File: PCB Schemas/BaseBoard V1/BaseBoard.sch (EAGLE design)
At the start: 31 parts, among them IC1 74HC595D, IC2 74HC595D, IC3 74HC595D, U1 ATMEGA2560AU, X1 16MHz

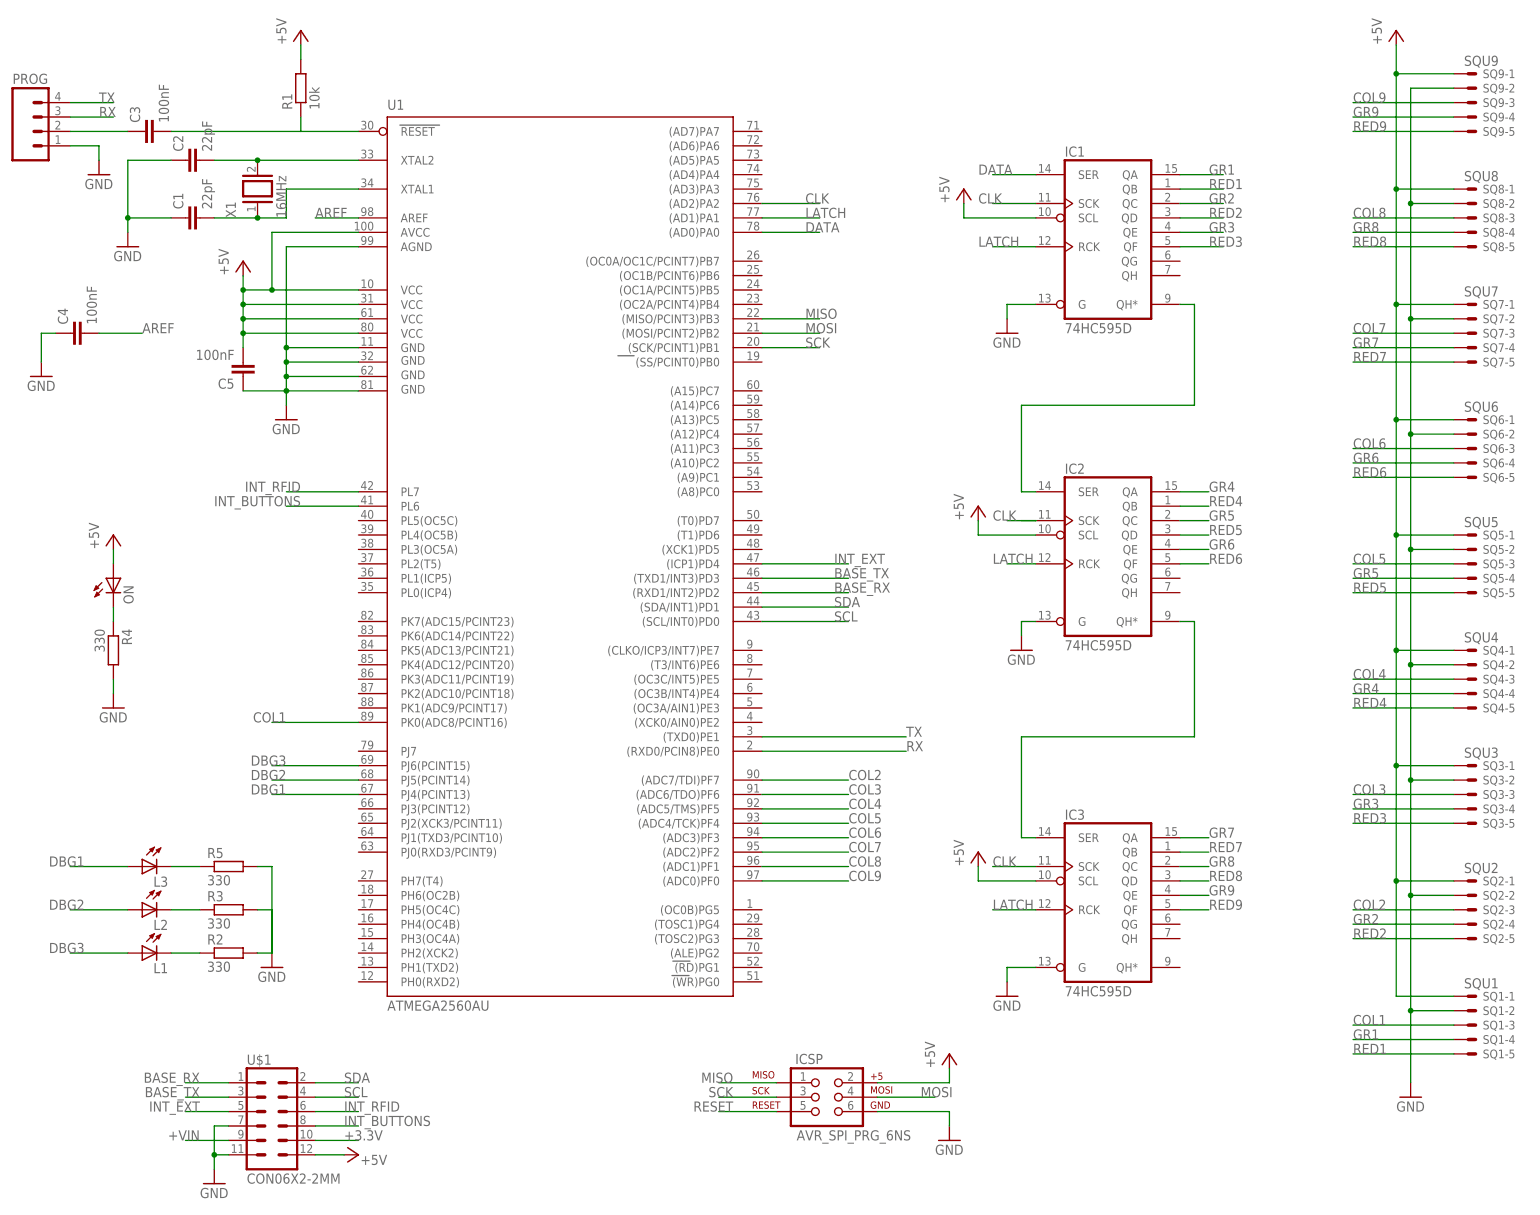
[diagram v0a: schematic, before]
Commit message: Updated details
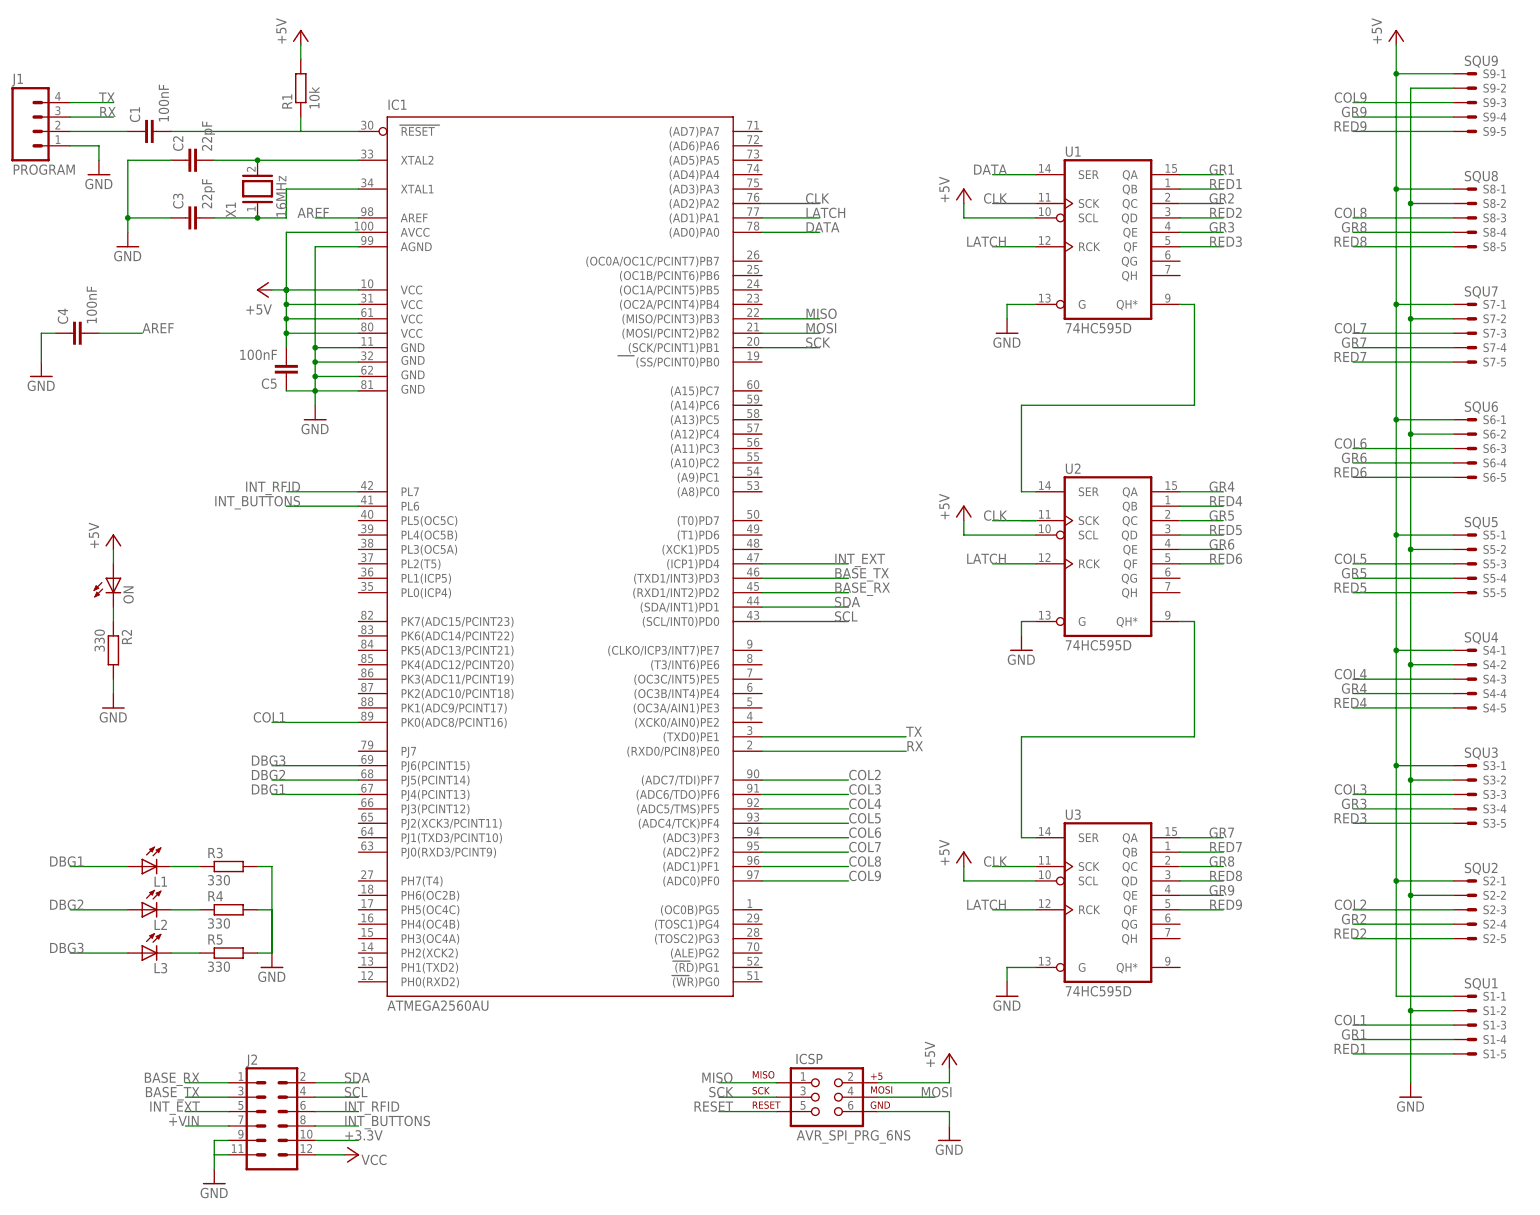
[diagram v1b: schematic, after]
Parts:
- C1: value 22pF -> 100nF
- C3: value 100nF -> 22pF
- IC1: value 74HC595D -> ATMEGA2560AU; device 74xx-eu:74HC595D -> SparkFun-DigitalIC:ATMEGA2560AU
- J1: value (none) -> PROGRAM
- U1: value ATMEGA2560AU -> 74HC595D; device SparkFun-DigitalIC:ATMEGA2560AU -> 74xx-eu:74HC595D
- renumbered IC2 to U2, IC3 to U3, PROG to J1, SQ1 to S1, SQ2 to S2, SQ3 to S3, SQ4 to S4, SQ5 to S5, SQ6 to S6, SQ7 to S7, SQ8 to S8, SQ9 to S9, U$1 to J2
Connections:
- removed net N$4 (its old number): L1.C, R2.1
- new net N$9: L1.C, R3.1
- net +VIN: now also J2.7; no longer J2.9
- net AREF: now also IC1.AREF; no longer U1.AREF
- net BASE_RX: now also IC1.(RXD1/INT2)PD2; no longer U1.(RXD1/INT2)PD2
- net BASE_TX: now also IC1.(TXD1/INT3)PD3; no longer U1.(TXD1/INT3)PD3
- net CLK: now also IC1.(AD2)PA2, U1A.SCK; no longer IC1A.SCK, U1.(AD2)PA2
- net COL1: now also IC1.PK0(ADC8/PCINT16); no longer U1.PK0(ADC8/PCINT16)
- net COL2: now also IC1.(ADC7/TDI)PF7; no longer U1.(ADC7/TDI)PF7
- net COL3: now also IC1.(ADC6/TDO)PF6; no longer U1.(ADC6/TDO)PF6
- net COL4: now also IC1.(ADC5/TMS)PF5; no longer U1.(ADC5/TMS)PF5
- net COL5: now also IC1.(ADC4/TCK)PF4; no longer U1.(ADC4/TCK)PF4
- net COL6: now also IC1.(ADC3)PF3; no longer U1.(ADC3)PF3
- net COL7: now also IC1.(ADC2)PF2; no longer U1.(ADC2)PF2
- net COL8: now also IC1.(ADC1)PF1; no longer U1.(ADC1)PF1
- net COL9: now also IC1.(ADC0)PF0; no longer U1.(ADC0)PF0
- net DATA: now also IC1.(AD0)PA0, U1A.SER; no longer IC1A.SER, U1.(AD0)PA0
- net DBG1: now also IC1.PJ4(PCINT13), L1.A; no longer L3.A, U1.PJ4(PCINT13)
- net DBG2: now also IC1.PJ5(PCINT14); no longer U1.PJ5(PCINT14)
- net DBG3: now also IC1.PJ6(PCINT15), L3.A; no longer L1.A, U1.PJ6(PCINT15)
- net GND: now also C3.1, IC1.AGND, IC1.GND, IC1.GND1, IC1.GND2, IC1.GND3, J2.9, U1A.G; no longer C1.1, IC1A.G, J2.7, U1.AGND, U1.GND, U1.GND1, U1.GND2, U1.GND3
- net GR1: now also U1A.QA; no longer IC1A.QA
- net GR2: now also U1A.QC; no longer IC1A.QC
- net GR3: now also U1A.QE; no longer IC1A.QE
- net INT_BUTTONS: now also IC1.PL6; no longer U1.PL6
- net INT_EXT: now also IC1.(ICP1)PD4; no longer U1.(ICP1)PD4
- net INT_RFID: now also IC1.PL7; no longer U1.PL7
- net LATCH: now also IC1.(AD1)PA1, U1A.RCK; no longer IC1A.RCK, U1.(AD1)PA1
- net MISO: now also IC1.(MISO/PCINT3)PB3; no longer U1.(MISO/PCINT3)PB3
- net MOSI: now also IC1.(MOSI/PCINT2)PB2; no longer U1.(MOSI/PCINT2)PB2
- net N$1: now also IC1.XTAL2; no longer U1.XTAL2
- net N$2: now also C3.2, IC1.XTAL1; no longer C1.2, U1.XTAL1
- net N$3: now also R4.1; no longer R3.1
- net N$5: now also C1.1; no longer C3.1
- net N$6: now also U1A.QH*; no longer IC1A.QH*
- net N$8: now also R2.1; no longer R4.1
- net RED1: now also U1A.QB; no longer IC1A.QB
- net RED2: now also U1A.QD; no longer IC1A.QD
- net RED3: now also U1A.QF; no longer IC1A.QF
- net RESET: now also C1.2, IC1.RESET; no longer C3.2, U1.RESET
- net RX: now also IC1.(RXD0/PCIN8)PE0; no longer U1.(RXD0/PCIN8)PE0
- net SCK: now also IC1.(SCK/PCINT1)PB1; no longer U1.(SCK/PCINT1)PB1
- net SCL: now also IC1.(SCL/INT0)PD0; no longer U1.(SCL/INT0)PD0
- net SDA: now also IC1.(SDA/INT1)PD1; no longer U1.(SDA/INT1)PD1
- net TX: now also IC1.(TXD0)PE1; no longer U1.(TXD0)PE1
- net VCC: now also IC1.AVCC, IC1.VCC, IC1.VCC1, IC1.VCC2, IC1.VCC3, U1A.SCL; no longer IC1A.SCL, U1.AVCC, U1.VCC, U1.VCC1, U1.VCC2, U1.VCC3
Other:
- moved on the sheet: C1, C3, C5, L1, L3, R2, R3, R4, R5
